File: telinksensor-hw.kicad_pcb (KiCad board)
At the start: 4 copper layers, 44 x 33.5 mm, 81 parts, among them J1 ANT, J2 3W RTD, J4 RTD 2W, J5 SOIC bite, Q1 2N7002, SW1 SW_Push, U1 TLSR8258, U2 SHT40, U3 BMP390, Y1 24MHz

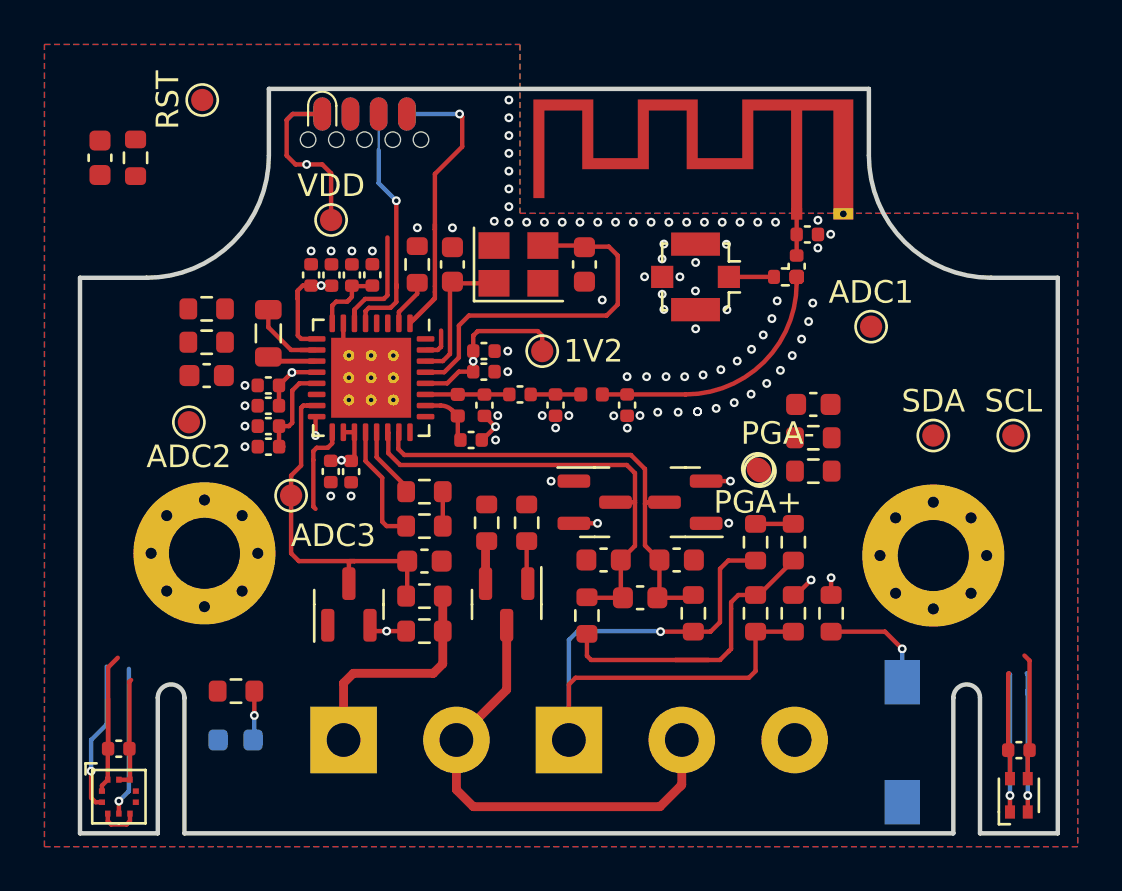
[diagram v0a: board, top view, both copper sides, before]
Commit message: Routing done
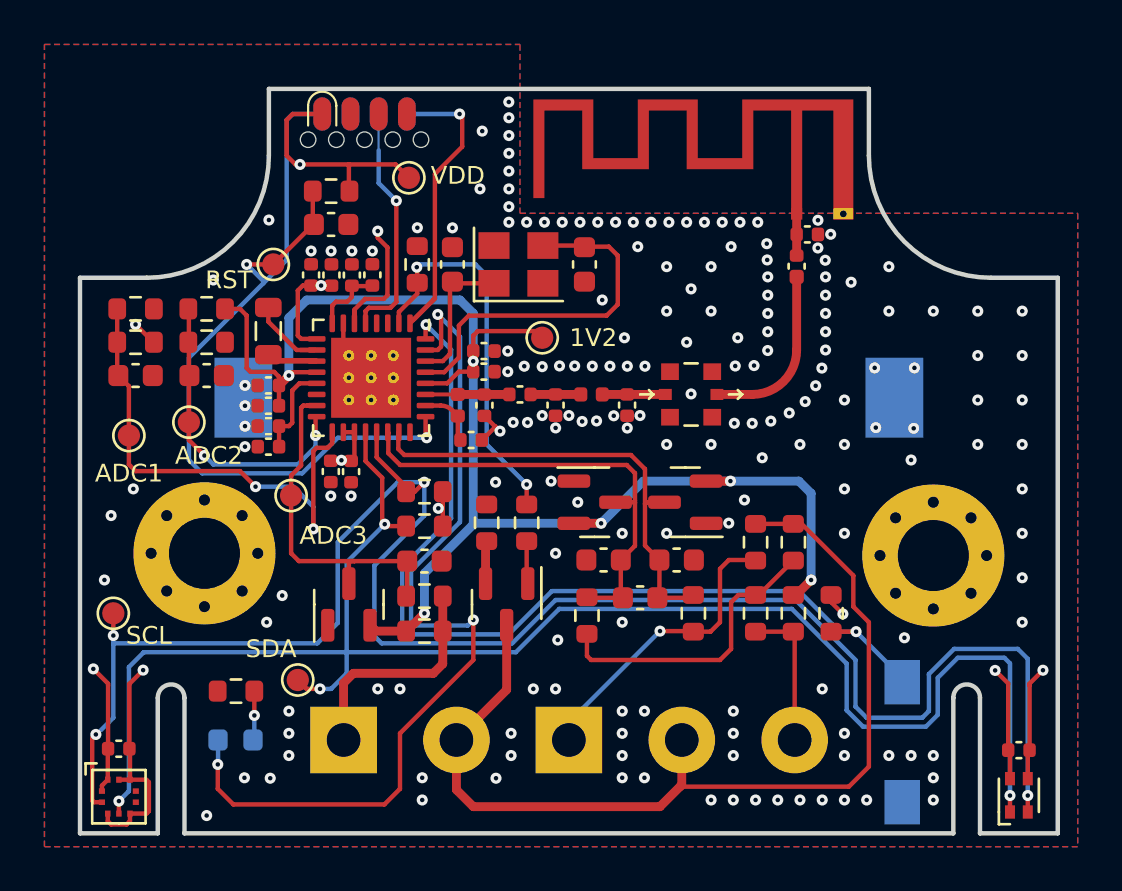
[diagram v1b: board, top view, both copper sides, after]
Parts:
- removed J1: ANT, Connector_Coaxial:U.FL_Molex_MCRF_73412-0110_Vertical
- removed R8: 0R, Resistor_SMD:R_0402_1005Metric
- removed TP1: PGA+, TestPoint:TestPoint_Pad_D1.0mm
- removed TP3: PGA-, TestPoint:TestPoint_Pad_D1.0mm
- added BT1: CR2032-BS-6-1, Battery:BatteryHolder_Keystone_1060_1x2032, B.Cu at (165.9, 97.4)
- added TP11: MM8130-2600, murrata:MM8130-2600, F.Cu at (171.4, 97.2)
- moved TP4 41.3 mm to (145.4, 107.1)
- moved TP7 33.8 mm to (146.1, 99.1), turned to 0 degrees
- moved R5 31.4 mm to (146.4, 93.4), turned to 0 degrees
- moved R4 30.8 mm to (146.4, 94.9), turned to 180 degrees
- moved TP5 30.6 mm to (153.7, 110.1)
- moved C11 30.5 mm to (146.4, 96.4), turned to 0 degrees
- moved C4 10.8 mm to (155.2, 89.6), turned to 0 degrees
- moved R1 8.93 mm to (155.2, 88.1), turned to 180 degrees
- moved TP2 8.06 mm to (152.6, 91.4), turned to 180 degrees
- moved TP10 3.98 mm to (158.7, 87.5)
- moved TP9 0.60 mm to (164.7, 94.7)
- moved L1 0.10 mm to (152.4, 94.4)
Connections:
- C18 pad 1: Net-(L3-Pad2) -> Net-(C18-Pad1)
- C20 pad 1: Net-(L3-Pad2) -> Net-(C20-Pad1)
- J2 pad 1: Net-(J2-Pad1) -> Net-(R10-Pad2)
- J2 pad 3: Net-(J2-Pad3) -> Net-(R13-Pad1)
- L3 pad 2: Net-(L3-Pad2) -> Net-(C20-Pad1)
- R10 pad 2: Net-(J2-Pad3) -> Net-(R10-Pad2)
- R13 pad 1: Net-(J2-Pad1) -> Net-(R13-Pad1)
- R15 pad 2: Net-(J2-Pad1) -> Net-(R13-Pad1)
- R17 pad 1: Net-(J2-Pad3) -> Net-(R10-Pad2)
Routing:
- net /SENSOR_PWR: track 21.2 -> 94.0 mm, vias 0 -> 4
- net /I2C_SCL: track 16.5 -> 83.3 mm, vias 2 -> 4
- net /I2C_SDA: track 18.5 -> 75.7 mm, vias 2 -> 4
- net +1V2: track 15.8 -> 68.0 mm
- net /LED: track 1.49 -> 40.4 mm, vias 0 -> 3
- net /BTN: track 5.02 -> 42.0 mm, vias 1 -> 2
- net /~{RST}: track 1.71 -> 37.9 mm, vias 0 -> 2
- net /GND_RTD: track 22.9 -> 44.3 mm
- net /ADC1: track 4.14 -> 22.3 mm, vias 0 -> 2
- net Net-(J2-Pad3): track 15.8 -> 0.00 mm, vias 1 -> 0
- net /RTD_ON: track 2.17 -> 17.5 mm, vias 0 -> 2
- net Net-(J2-Pad1): track 14.7 -> 0.00 mm
- net Net-(R10-Pad2): track 0.00 -> 13.7 mm, vias 0 -> 1
- net /ADC2: track 0.87 -> 13.8 mm, vias 1 -> 2
- net Net-(L3-Pad2): track 11.7 -> 0.00 mm
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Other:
- board text added: "JLCJLCJLCJLC"
- board text added: "RTD"
- board text added: "TSENSOR V1.0 18.11. 2022"
- board text added: "Vojtěch Vosáhlo"
